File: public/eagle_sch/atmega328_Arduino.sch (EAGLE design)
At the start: 10 parts, among them J2 ICSP, U3 ATMEGA328, Y1 16MHz

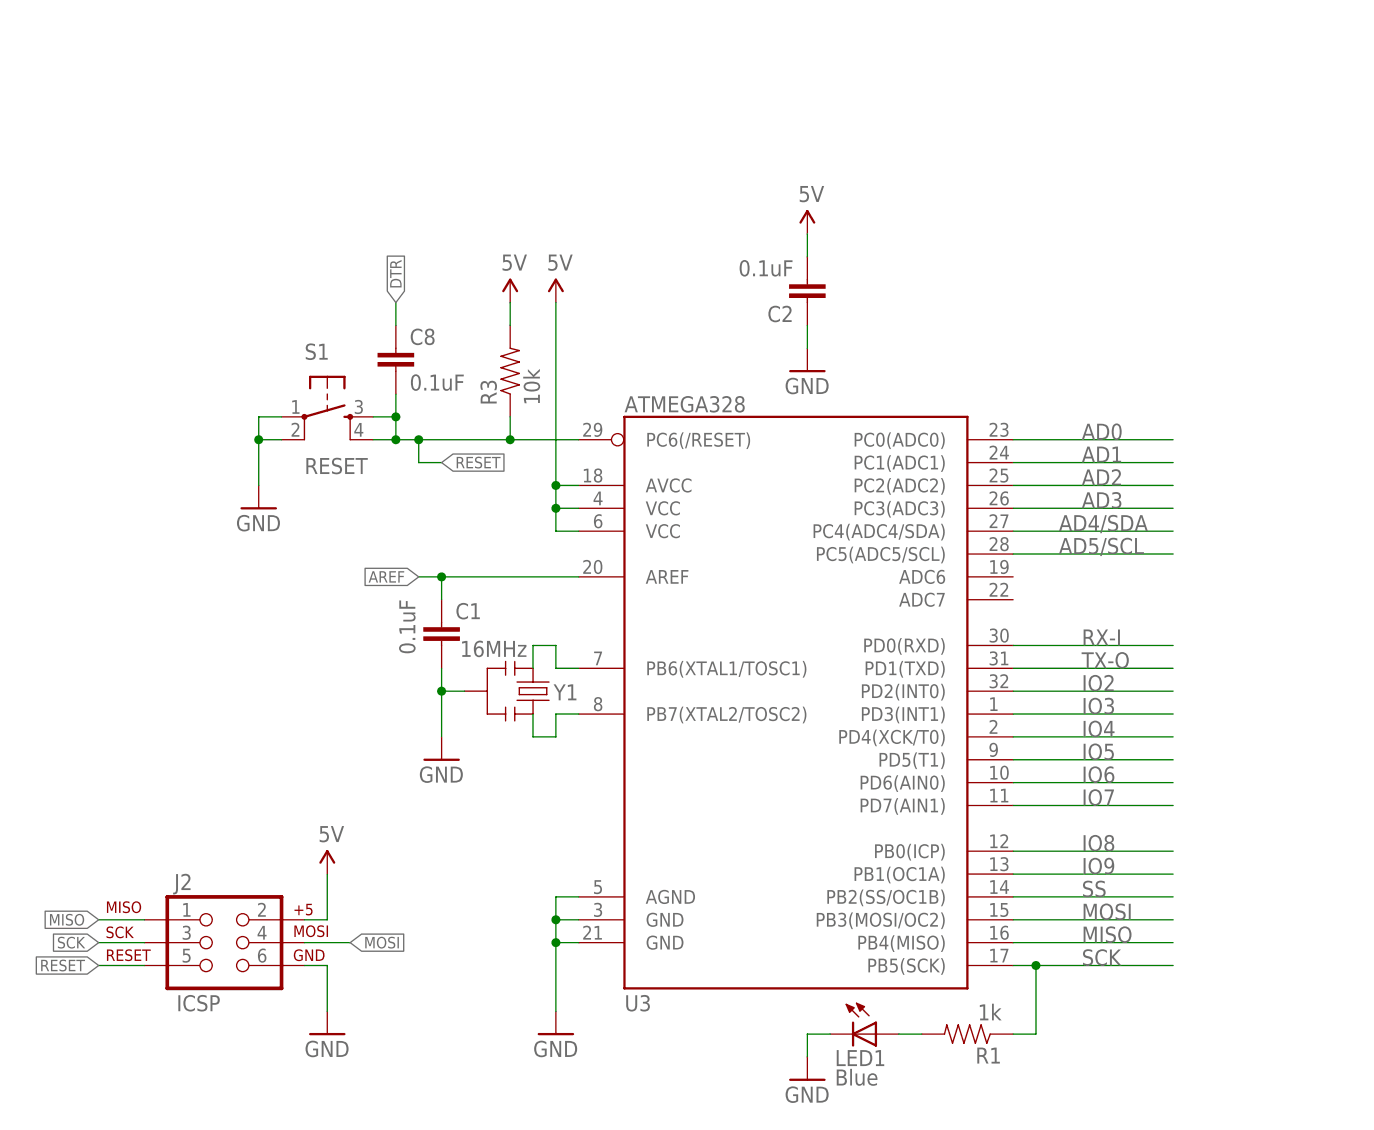
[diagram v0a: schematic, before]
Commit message: download sch
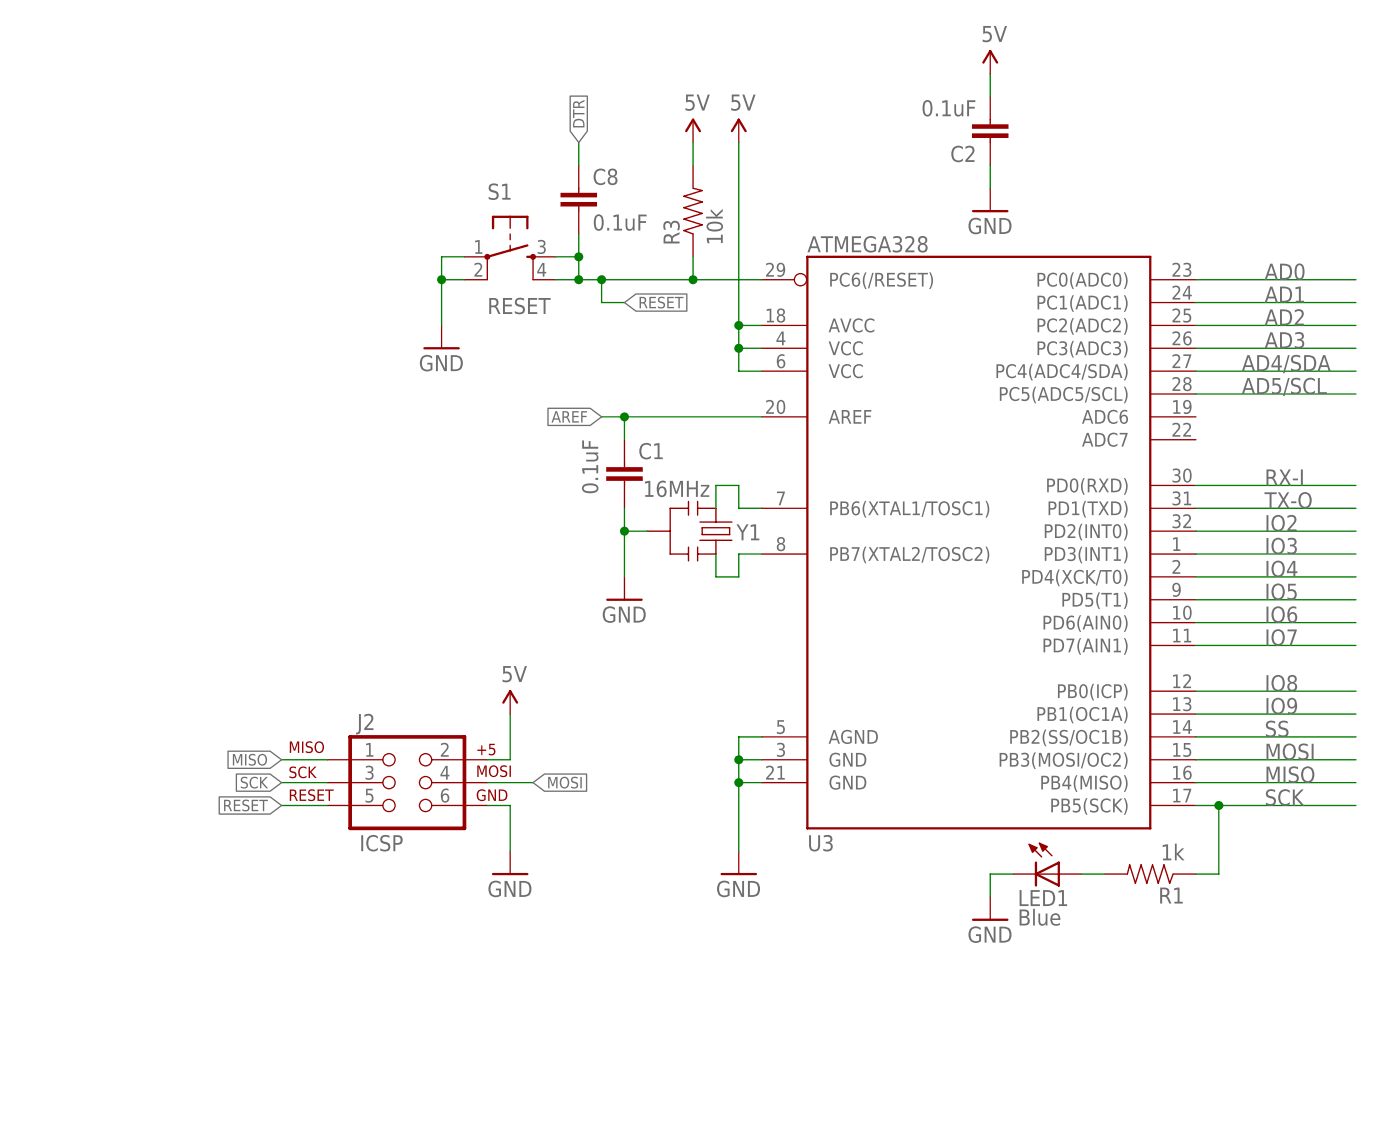
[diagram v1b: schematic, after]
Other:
- moved on the sheet: C1, C2, C8, J2, LED1, R1, R3, S1, U3, Y1
